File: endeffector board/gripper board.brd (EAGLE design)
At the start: 63.5 x 63.2 mm, 45 parts, among them J1 APPPP45_PCB_HORIZ_RIGHT, J2 APPPP45_PCB_HORIZ_RIGHT, J3 APPPP45_PCB_HORIZ_RIGHT, J4 APPPP45_PCB_HORIZ_RIGHT, J5 APPPP45_PCB_HORIZ_RIGHT, J6 SL03, Q1 MOSFET-NCHANNELFDD8780, U1 MAX232D

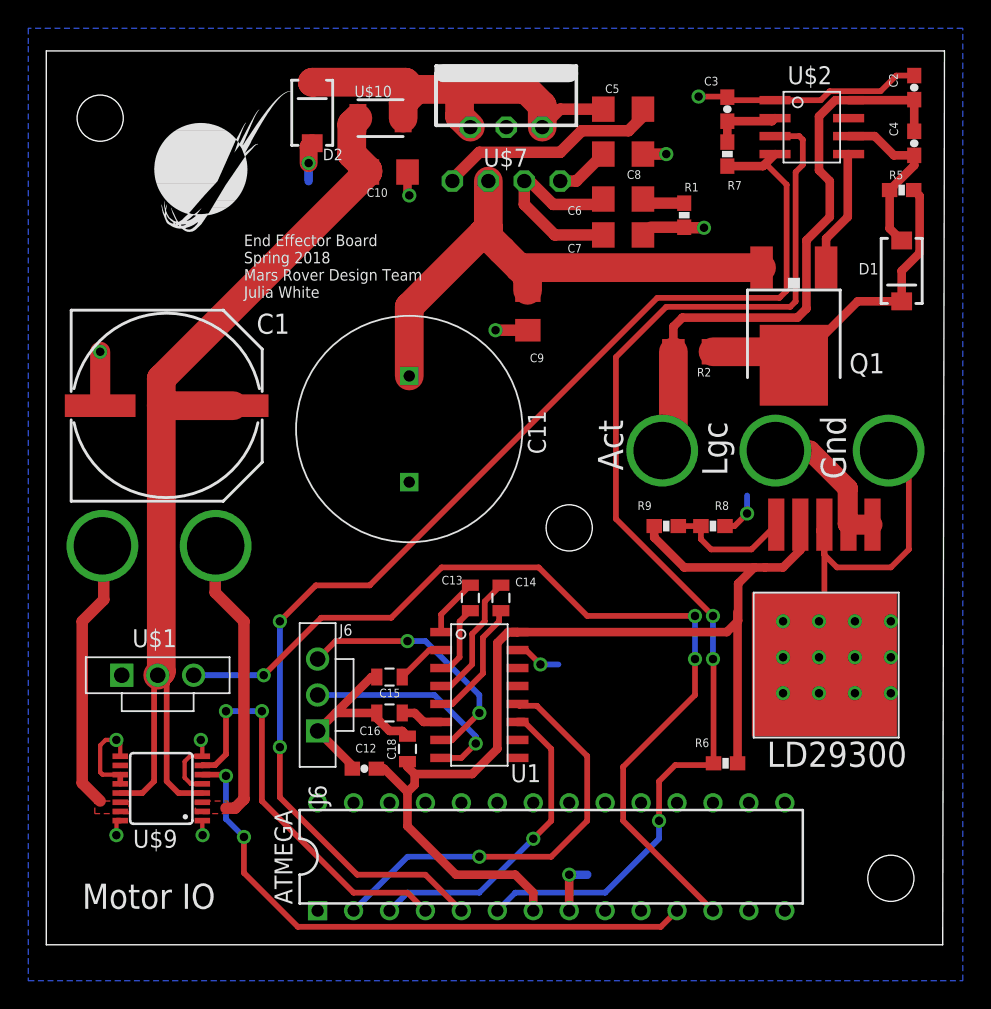
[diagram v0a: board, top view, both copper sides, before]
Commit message: Add files via upload
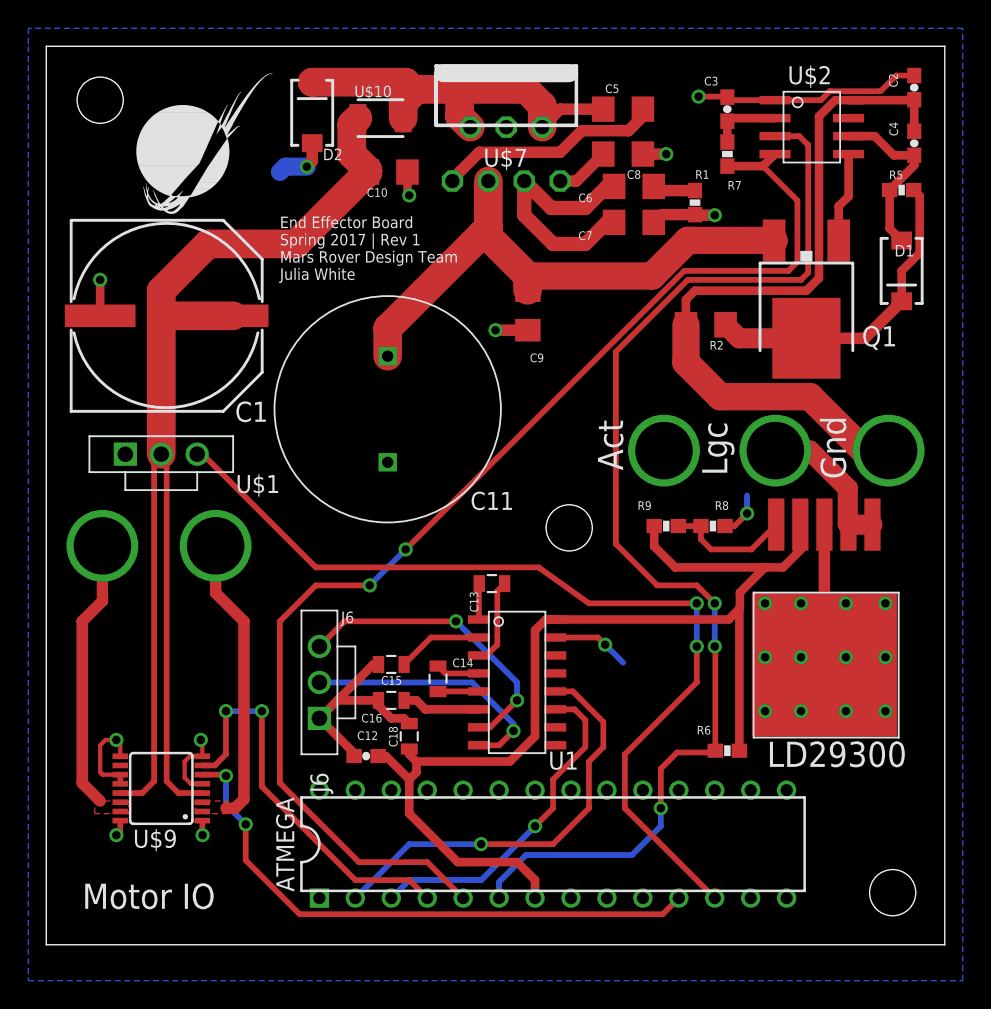
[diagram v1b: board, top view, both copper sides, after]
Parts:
- U$7: value SANC8050 -> SI-8050Y
- moved J3 16.0 mm to (63.5, 63.1)
- moved J1 15.9 mm to (47.6, 63.1)
- moved U$1 15.6 mm to (8.13, 34.7)
- moved C14 7.24 mm to (27.7, 18.8)
- moved C1 6.35 mm to (8.51, 44.5)
- moved U1 2.81 mm to (33.3, 18.5)
- moved R2 2.10 mm to (46.6, 43.8)
- moved Q1 2.10 mm to (53.7, 44.5)
- moved C11 2.07 mm to (24.1, 37.8)
- moved C13 1.83 mm to (31.5, 25.5), turned to 0 degrees
- moved LOGO1 1.80 mm to (6.35, 50.8)
- moved H2 1.27 mm to (3.81, 59.7)
- moved C6 1.17 mm to (41.5, 53.6)
- moved C7 1.17 mm to (41.5, 51.1)
- moved R1 1.17 mm to (45.8, 52.5)
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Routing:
- net 5VMTR: track 72.6 -> 91.8 mm
- net GND: track 99.6 -> 84.7 mm, vias 14 -> 25
- net ACTPWR: track 43.1 -> 52.3 mm
- net N$14: track 9.26 -> 3.10 mm
- net N$13: track 8.81 -> 2.89 mm
- net N$10: track 14.6 -> 18.4 mm
- net MICROCNTRL: track 90.2 -> 86.5 mm
- net N$18: track 18.3 -> 21.3 mm
- net N$19: track 15.8 -> 18.3 mm
- net N$17: track 3.01 -> 5.55 mm
- net N$16: track 3.54 -> 6.08 mm
- net N$9: track 24.8 -> 22.5 mm
- net N$7: track 8.68 -> 6.41 mm
- net N$15: track 4.17 -> 2.55 mm
- net ATMEGA2MAX: track 22.3 -> 23.7 mm
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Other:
- board size 63.5 x 63.2 mm -> 63.5 x 63.5 mm
- board text added: "End Effector Board Spring 2017 | Rev 1 Mars Rover Design Team Julia White"
- board text removed: "End Effector Board Spring 2018 Mars Rover Design Team Julia White"
